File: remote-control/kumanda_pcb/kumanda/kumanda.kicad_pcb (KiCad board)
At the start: 2 copper layers, 38 parts, among them J1 USB_A, J2 Conn_01x04, J3 RJ45, J4 Conn_01x06, J5 Screw_Terminal_01x02, U1 MEGA_PRO_EMBED_CH340G___ATMEG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

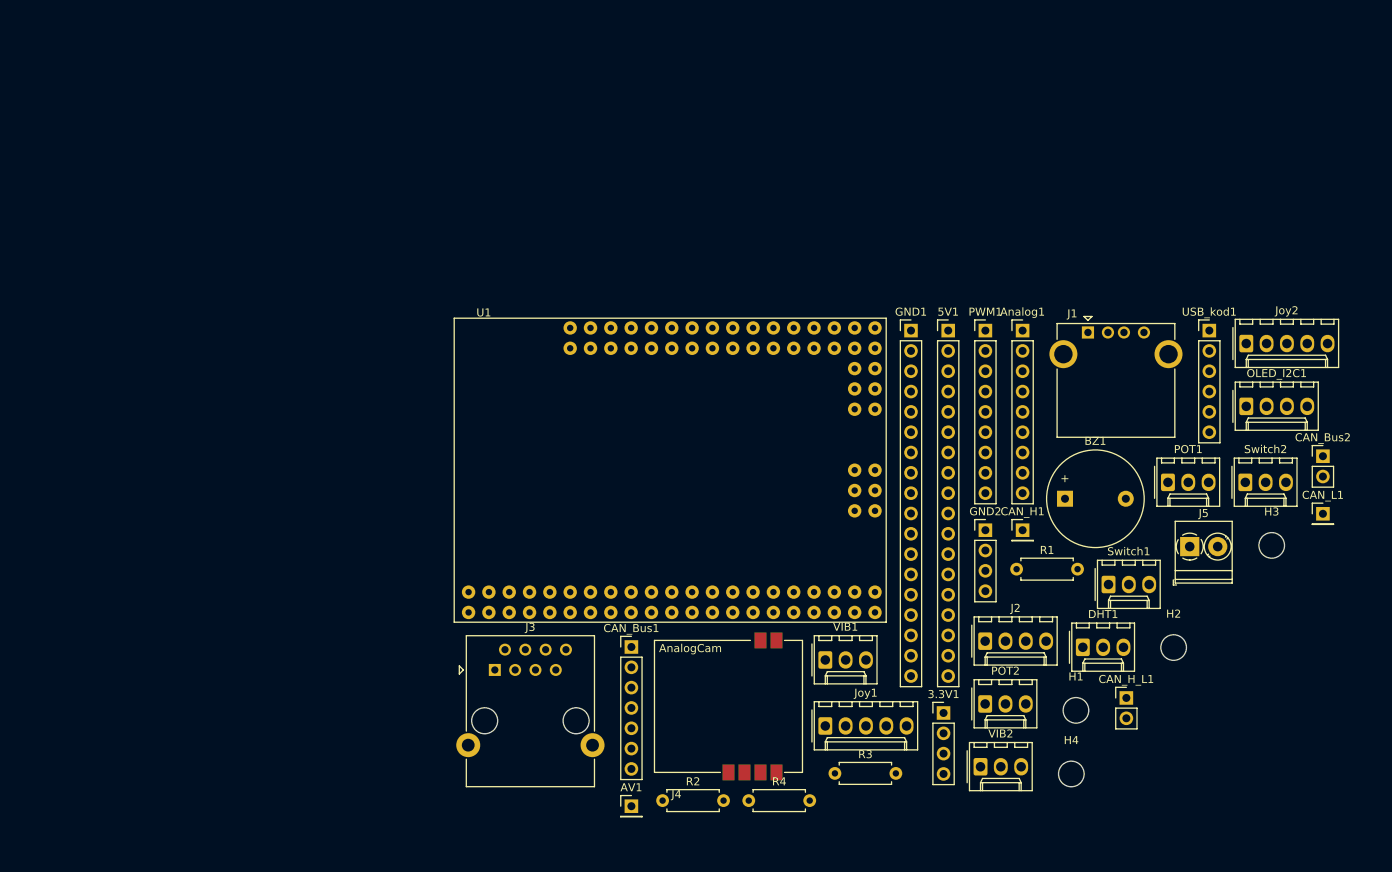
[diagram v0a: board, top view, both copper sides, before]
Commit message: PCB design finished.
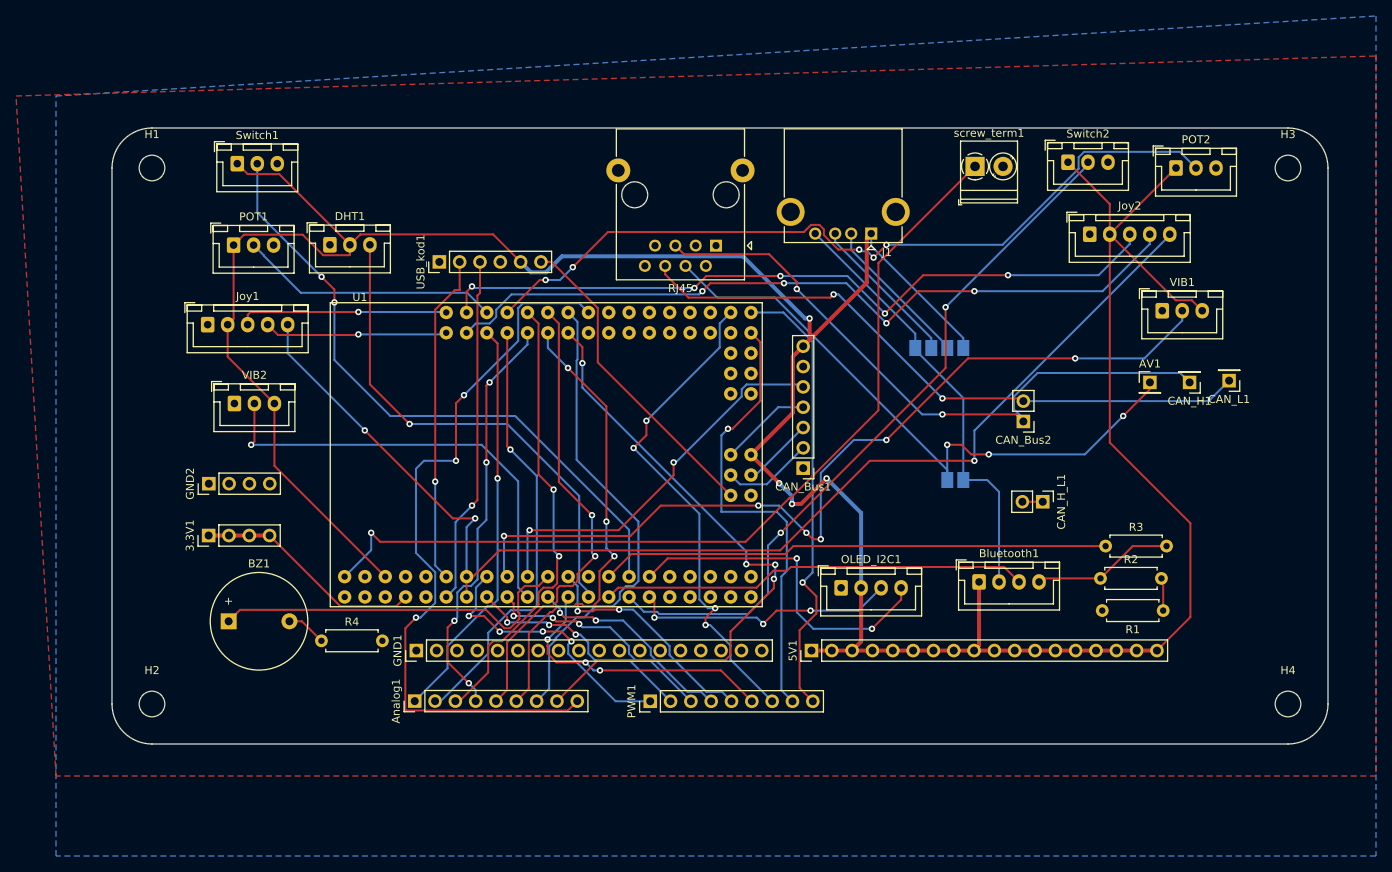
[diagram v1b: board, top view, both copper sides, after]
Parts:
- removed J2: Conn_01x04, Connector_Molex:Molex_KK-254_AE-6410-04A_1x04_P2.54mm_Vertical
- removed J3: RJ45, Connector_RJ:RJ45_Ninigi_GE
- removed J4: Conn_01x06, analog_cam:Analog-cam
- removed J5: Screw_Terminal_01x02, TerminalBlock_Phoenix:TerminalBlock_Phoenix_PT-1,5-2-3.5-H_1x02_P3.50mm_Horizontal
- added AV_conv1: Conn_01x06, analog_cam:Analog-cam, B.Cu at (152.7, 66.5)
- added Bluetooth1: Conn_01x04, Connector_JST:JST_XH_B4B-XH-A_1x04_P2.50mm_Vertical, F.Cu at (160.4, 95.7)
- added RJ45: RJ45, Connector_RJ:RJ45_Ninigi_GE, F.Cu at (127.5, 53.7)
- added screw_term1: Screw_Terminal_01x02, TerminalBlock_Phoenix:TerminalBlock_Phoenix_PT-1,5-2-3.5-H_1x02_P3.50mm_Horizontal, F.Cu at (159.9, 43.8)
- DHT1, POT1, POT2, Switch1, Switch2, VIB1, VIB2: footprint Connector_Molex:Molex_KK-254_AE-6410-03A_1x03_P2.54mm_Vertical -> Connector_JST:JST_XH_B3B-XH-A_1x03_P2.50mm_Vertical
- Joy1, Joy2: footprint Connector_Molex:Molex_KK-254_AE-6410-05A_1x05_P2.54mm_Vertical -> Connector_JST:JST_XH_B5B-XH-A_1x05_P2.50mm_Vertical
- OLED_I2C1: footprint Connector_Molex:Molex_KK-254_AE-6410-04A_1x04_P2.54mm_Vertical -> Connector_JST:JST_XH_B4B-XH-A_1x04_P2.50mm_Vertical
- U1: footprint MODULE_MEGA_PRO_EMBED_CH340G_git:_ATMEGA2560 -> MODULE_MEGA_PRO_EMBED_CH340G_:_ATMEGA2560
- moved H1 133.9 mm to (57.0, 44.0)
- moved H2 127.9 mm to (57.0, 111.0)
- moved Switch1 120.9 mm to (67.7, 43.5)
- moved POT1 120.5 mm to (67.2, 53.6)
- moved DHT1 106.7 mm to (79.2, 53.6)
- moved BZ1 105.7 mm to (66.6, 100.7)
- moved VIB2 103.7 mm to (67.3, 73.4)
- moved GND2 97.2 mm to (64.1, 83.5), turned to 90 degrees
- moved USB_kod1 96.6 mm to (92.9, 55.7), turned to 90 degrees
- moved 3.3V1 94.5 mm to (64.1, 89.9), turned to 90 degrees
- moved Joy1 92.1 mm to (64.0, 63.6)
- moved Analog1 89.0 mm to (89.8, 110.6), turned to 90 degrees
- moved AV1 83.7 mm to (181.7, 70.8)
- moved GND1 73.6 mm to (90.0, 104.3), turned to 90 degrees
- moved POT2 71.1 mm to (185.0, 44.0)
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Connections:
- U1 pad RX: Net-(U1-PadRX) -> RX
- U1 pad TX: Net-(U1-PadTX) -> TX
- USB_kod1 pad 5: 5v -> VBUS
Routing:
- net VBUS: track 0.00 -> 392.4 mm, vias 0 -> 4
- net /SW: track 0.00 -> 153.3 mm, vias 0 -> 3
- net /A0: track 0.00 -> 119.4 mm, vias 0 -> 6
- net /A1: track 0.00 -> 118.9 mm, vias 0 -> 5
- net VIN: track 0.00 -> 113.0 mm, vias 0 -> 1
- net /D6: track 0.00 -> 110.7 mm, vias 0 -> 6
- net /A6: track 0.00 -> 99.9 mm, vias 0 -> 5
- net TX: track 0.00 -> 97.2 mm, vias 0 -> 1
- net A14: track 0.00 -> 92.3 mm, vias 0 -> 3
- net /D19: track 0.00 -> 89.8 mm, vias 0 -> 2
- net /CAN_H: track 0.00 -> 80.4 mm, vias 0 -> 2
- net /D18: track 0.00 -> 80.0 mm, vias 0 -> 2
- net /CAN_L: track 0.00 -> 79.5 mm, vias 0 -> 2
- net A13: track 0.00 -> 79.5 mm, vias 0 -> 4
- net AV: track 0.00 -> 79.0 mm, vias 0 -> 3
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- added copper zone on B.Cu, net GND
- added copper zone on F.Cu, net GND
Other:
- board outline added: 152 x 77 mm
